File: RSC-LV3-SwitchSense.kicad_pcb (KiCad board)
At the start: 2 copper layers, 159 parts, among them J1 FTSH-105-01-L-DV-K-A, J10 Molex 43045-0400, J11 Molex 43045-0400, J12 Molex 43045-0400, J13 Molex 43045-0400, J14 Molex 43045-0400, J15 Molex 43045-0400, J2 USB_C_Receptacle_USB2.0_16P, J3 Molex 43650-0500, J4 Molex 43650-0500, J6 Molex 43045-0400, J7 Molex 43045-0400, J8 Molex 43045-0400, J9 Molex 43045-0400, Q1 AO3400A, Q10 AO3400A, Q2 AO3400A, Q3 AO3400A, Q4 AO3400A, Q5 AO3400A, Q6 AO3400A, Q7 AO3400A, Q8 AO3400A, Q9 AO3400A, U1 STM32G0B1CBTx, U2 TPS54302, U3 TLV74033PDBVR, U4 TJA1051T-3, Y1 Crystal_GND24

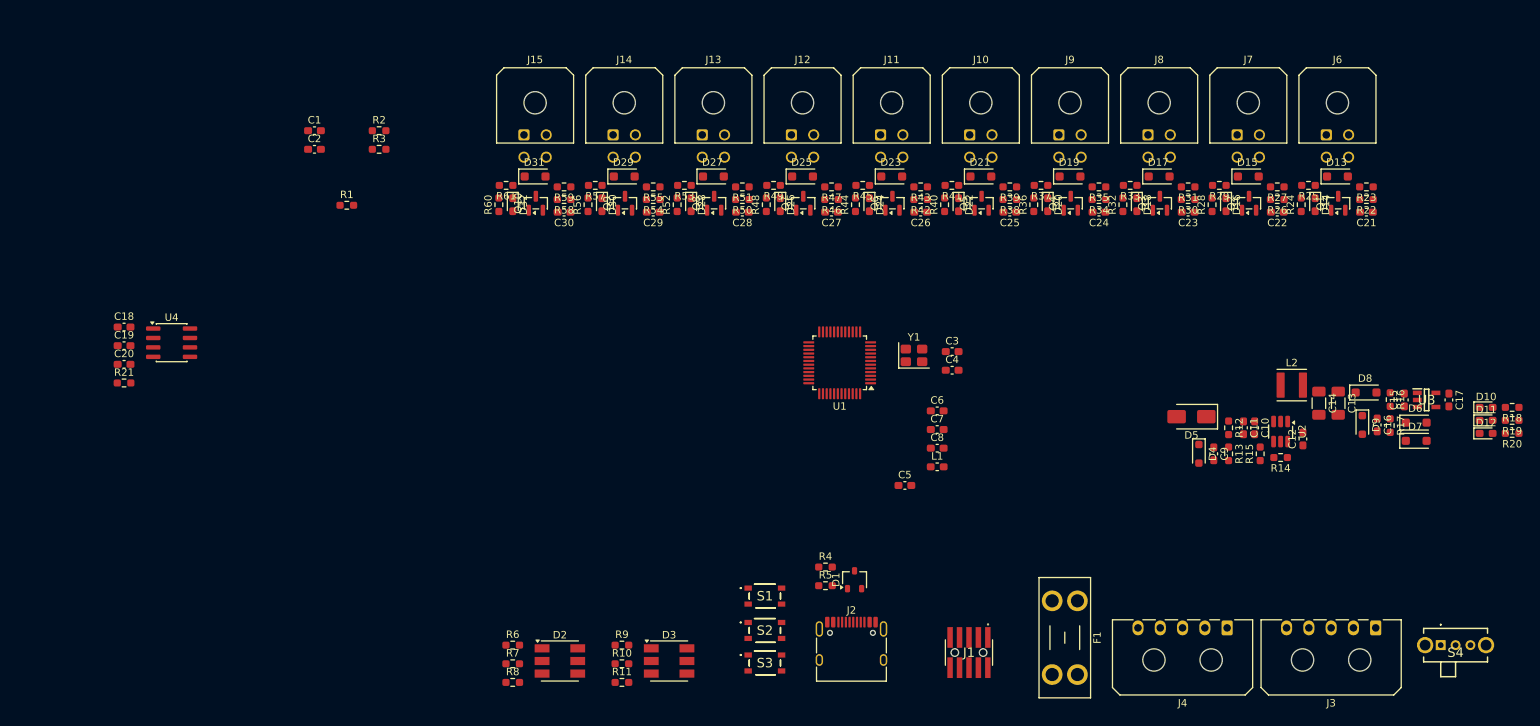
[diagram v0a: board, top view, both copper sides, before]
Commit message: more layout work
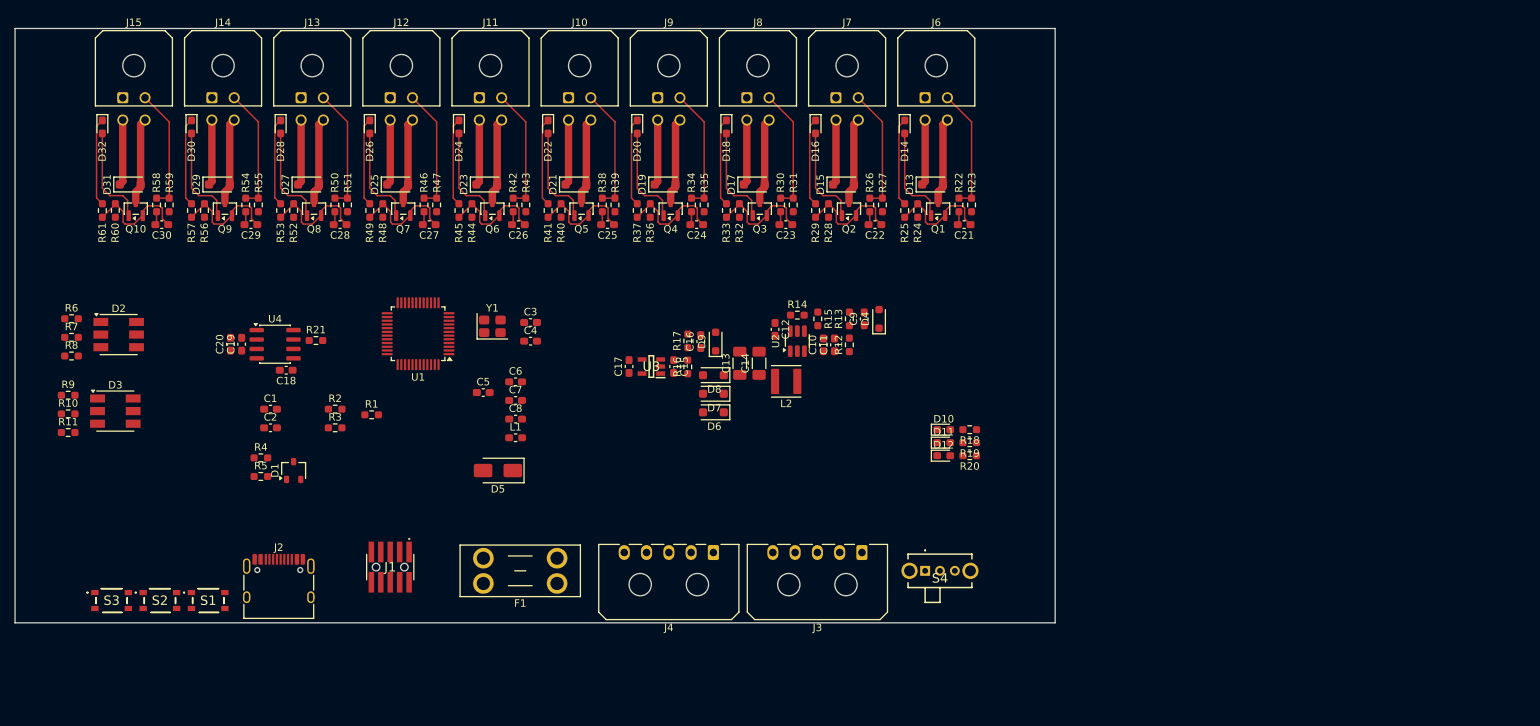
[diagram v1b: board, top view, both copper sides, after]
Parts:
- moved C17 110.4 mm to (152.7, 95.5), turned to 90 degrees
- moved U3 104.4 mm to (155.7, 95.5), turned to 180 degrees
- moved C15 98.5 mm to (158.7, 95.5), turned to -90 degrees
- moved R17 95.2 mm to (160.6, 92.0), turned to 90 degrees
- moved D7 94.8 mm to (164.0, 99.2), turned to 180 degrees
- moved R16 94.7 mm to (160.6, 95.5), turned to 90 degrees
- moved D6 94.6 mm to (164.0, 101.7), turned to 180 degrees
- moved D5 93.6 mm to (135.0, 109.5)
- moved C16 91.7 mm to (162.3, 92.1), turned to 90 degrees
- moved S3 88.3 mm to (83.0, 127.0)
- moved D8 87.9 mm to (164.0, 96.7), turned to 180 degrees
- moved D9 87.8 mm to (164.3, 92.1), turned to 90 degrees
- moved D3 81.8 mm to (83.5, 101.5)
- moved R10 81.8 mm to (77.2, 101.9)
- moved R11 81.8 mm to (77.2, 104.4)
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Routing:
- net GND: track 0.00 -> 150.3 mm
- net +12V: track 0.00 -> 88.5 mm
- net Net-(J15-Pin_2): track 0.00 -> 16.6 mm
- net Net-(J14-Pin_2): track 0.00 -> 16.6 mm
- net Net-(J13-Pin_2): track 0.00 -> 16.6 mm
- net Net-(J12-Pin_2): track 0.00 -> 16.6 mm
- net Net-(J9-Pin_2): track 0.00 -> 16.6 mm
- net Net-(J8-Pin_2): track 0.00 -> 16.6 mm
- net Net-(J7-Pin_2): track 0.00 -> 16.6 mm
- net Net-(J6-Pin_2): track 0.00 -> 16.6 mm
- net Net-(J11-Pin_2): track 0.00 -> 16.6 mm
- net Net-(J10-Pin_2): track 0.00 -> 16.6 mm
- net OUT_6: track 0.00 -> 13.6 mm
- net OUT_5: track 0.00 -> 13.6 mm
- net OUT_4: track 0.00 -> 13.6 mm
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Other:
- board outline added: 140 x 80 mm
